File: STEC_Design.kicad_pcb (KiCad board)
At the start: 2 copper layers, 13 parts, among them Q1 IRLB3034PBF, Q2 IRLB3034PBF, SW1 SW_Push (Down), SW2 SW_Push (Up), U1 L7805CV, U2 MLX90614ESF-BAA-000-TU, U4 ESP32-DEVKITC-32E

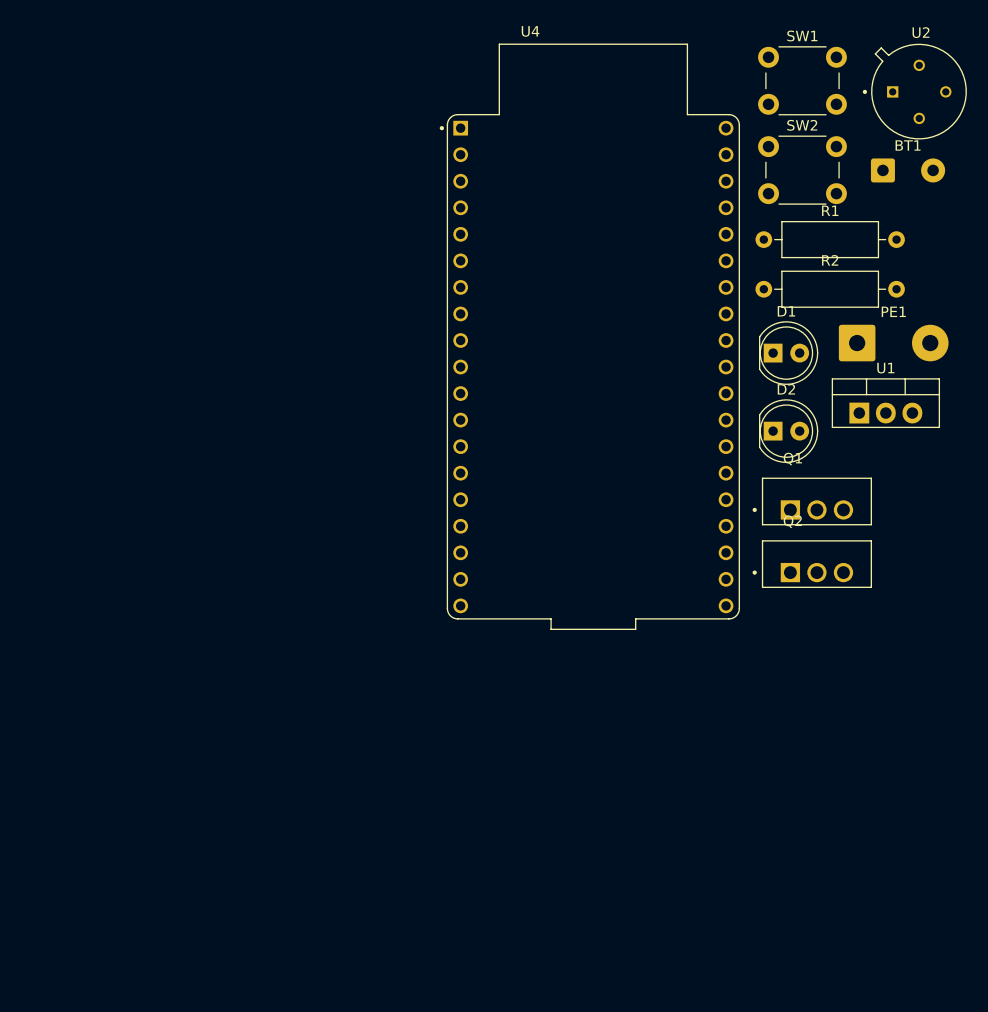
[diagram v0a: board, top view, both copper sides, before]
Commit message: finishedPCBdesign
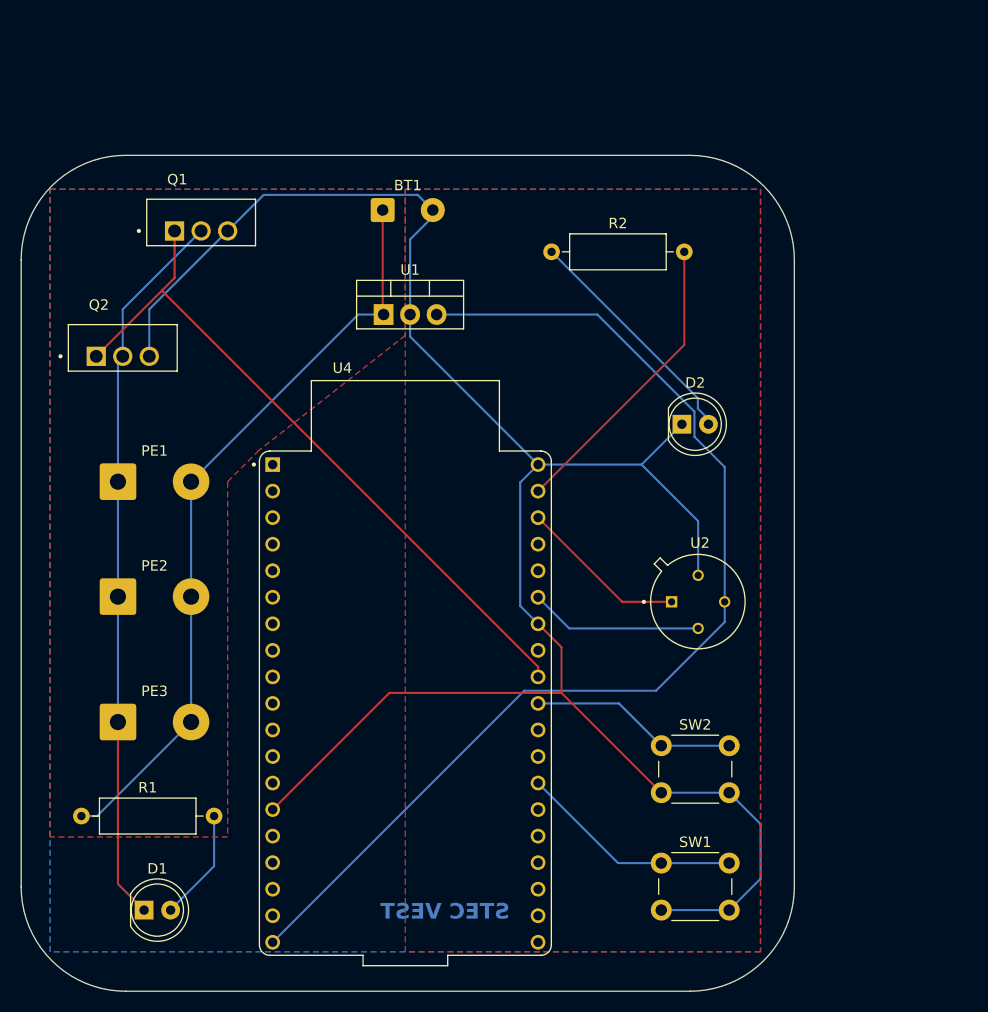
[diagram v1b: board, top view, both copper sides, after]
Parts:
- added PE2: TEC, Connector_Wire:SolderWire-0.75sqmm_1x02_P7mm_D1.25mm_OD3.5mm, F.Cu at (118.5, 100.0)
- added PE3: TEC, Connector_Wire:SolderWire-0.75sqmm_1x02_P7mm_D1.25mm_OD3.5mm, F.Cu at (118.5, 112.0)
- D2: value WiFi_LED -> WiFi_LED (Red)
- PE1: value TEC(x3) -> TEC
- moved R1 85.5 mm to (115.0, 121.0)
- moved D1 80.4 mm to (121.0, 130.0)
- moved SW1 77.8 mm to (170.5, 125.5)
- moved PE1 72.0 mm to (118.5, 89.0)
- moved Q2 69.6 mm to (119.0, 76.2)
- moved Q1 64.7 mm to (126.5, 64.2)
- moved SW2 58.2 mm to (170.5, 114.3)
- moved U2 53.2 mm to (174.0, 100.5)
- moved BT1 48.0 mm to (143.8, 63.0)
- moved U1 46.5 mm to (143.9, 73.0)
- moved U4 36.9 mm to (146.0, 110.2)
- moved R2 20.6 mm to (160.0, 67.0)
- moved D2 8.75 mm to (172.5, 83.5)
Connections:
- net Net-(U1-OUT) renamed +5V
- Q1 pad 2: GND -> Net-(D1-K)
- Q1 pad 3: Net-(D1-K) -> GND
- Q2 pad 2: GND -> Net-(D1-K)
- Q2 pad 3: Net-(D1-K) -> GND
- U4 pad J2_14: unconnected-(U4-GND_J2_14-PadJ2_14) -> GND
- U4 pad J3_1: unconnected-(U4-GND_J3_1-PadJ3_1) -> GND
- U4 pad J3_7: unconnected-(U4-GND_J3_7-PadJ3_7) -> GND
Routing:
- net GND: track 0.00 -> 192.0 mm
- net +5V: track 0.00 -> 105.8 mm
- net +12V: track 0.00 -> 72.3 mm
- net Net-(D1-K): track 0.00 -> 69.8 mm
- net Net-(Q1-G): track 0.00 -> 67.0 mm
- net Net-(U4-IO23): track 0.00 -> 28.7 mm
- net Net-(D2-A): track 0.00 -> 22.7 mm
- net Net-(U4-IO4): track 0.00 -> 21.5 mm
- net Net-(U4-IO5): track 0.00 -> 20.0 mm
- net Net-(U2-SCL/VZ): track 0.00 -> 16.7 mm
- net Net-(U2-SDA/PWM): track 0.00 -> 16.6 mm
- net Net-(D1-A): track 0.00 -> 10.7 mm
- added copper zone on F.Cu, net +12V
- added copper zone on F.Cu, net +5V
- added copper zone on B.Cu, net GND
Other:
- board outline added: 74 x 80 mm
- board text added: "STEC VEST"
